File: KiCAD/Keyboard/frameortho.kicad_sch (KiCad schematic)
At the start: 1 part, among them U1 RP2040

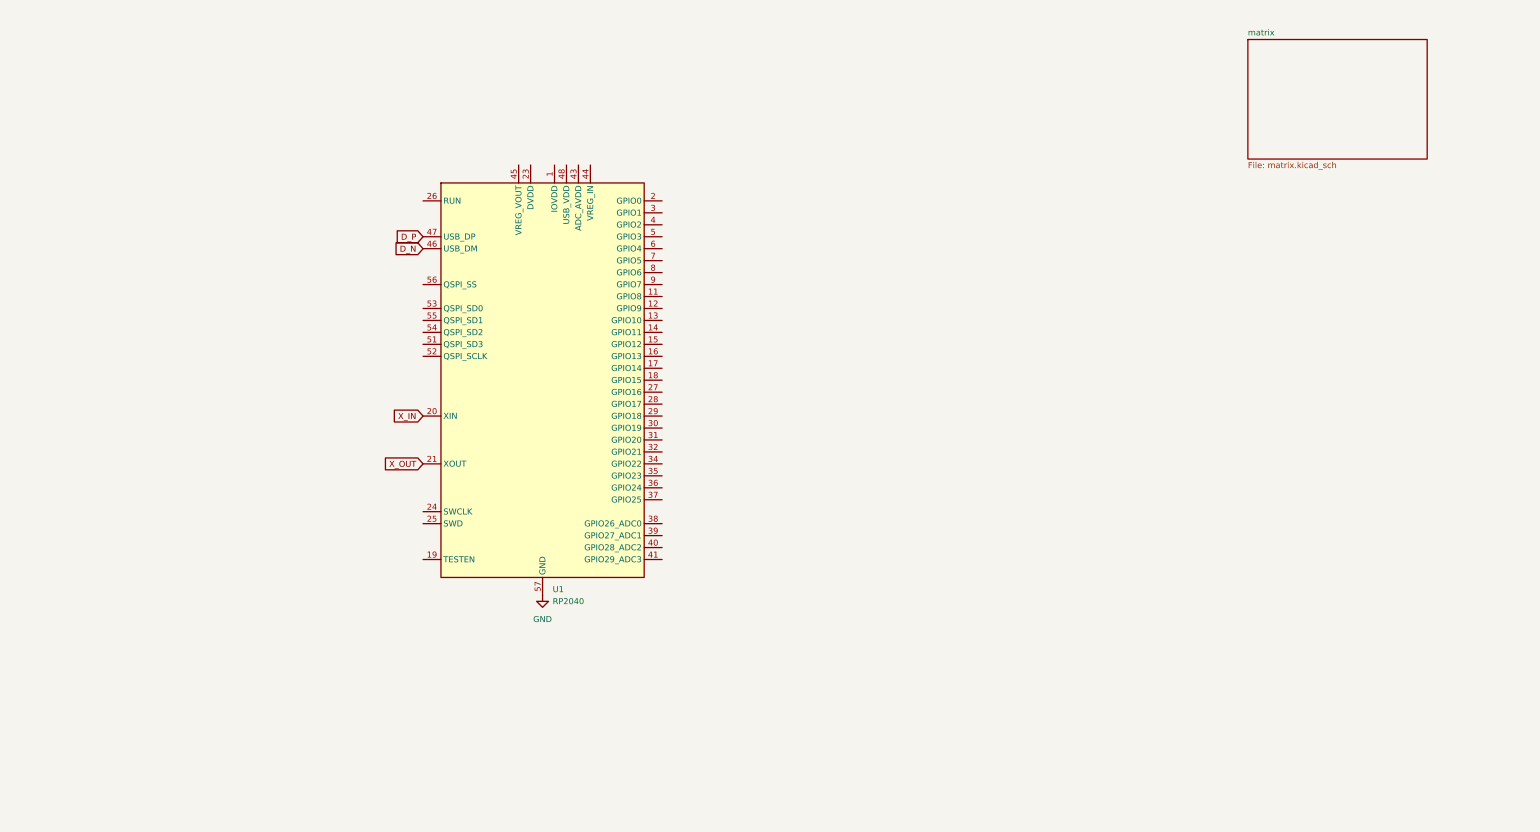
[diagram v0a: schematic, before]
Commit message: start keyboard pcb
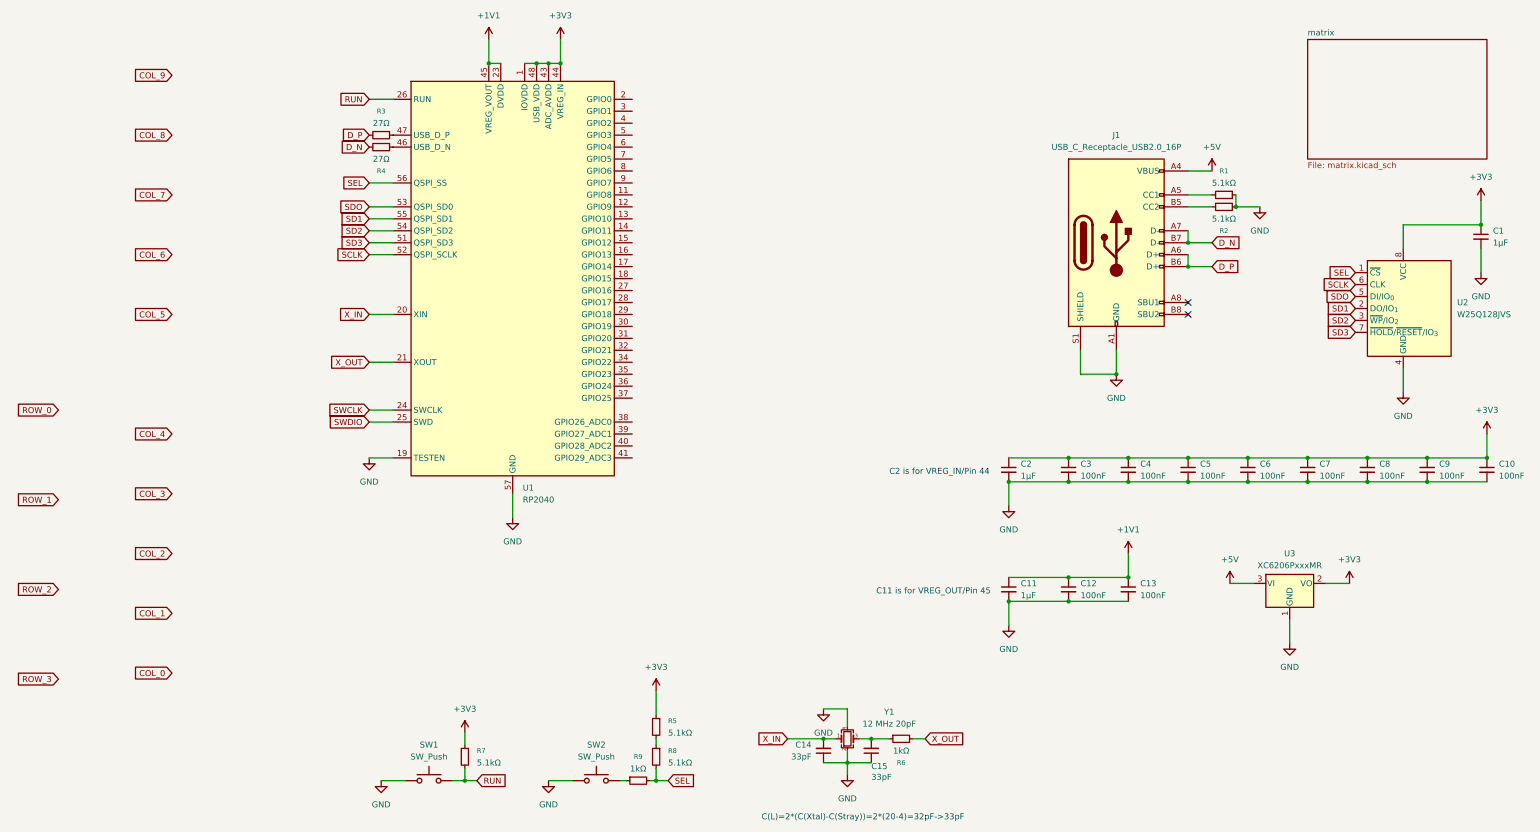
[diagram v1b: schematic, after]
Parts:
- added C1, C11, C2: 1µF, Capacitor_SMD:C_0402_1005Metric, symbol Device:C_Small
- added C10, C12, C13, C3, C4, C5, C6, C7, C8, C9: 100nF, Capacitor_SMD:C_0402_1005Metric, symbol Device:C_Small
- added C14, C15: 33pF, Capacitor_SMD:C_0402_1005Metric, symbol Device:C_Small
- added J1: USB_C_Receptacle_USB2.0_16P, ScottoKeebs_Components:USB_C_HRO_TYPE-C-31-M-14, symbol Connector:USB_C_Receptacle_USB2.0_16P
- added R1, R2, R5, R7, R8: 5.1kΩ, Resistor_SMD:R_0402_1005Metric, symbol Device:R_Small
- added R3, R4: 27Ω, Resistor_SMD:R_0402_1005Metric, symbol Device:R_Small
- added R6, R9: 1kΩ, Resistor_SMD:R_0402_1005Metric, symbol Device:R_Small
- added SW1, SW2: SW_Push, ScottoKeebs_Components:Button_TL3342, symbol Switch:SW_Push
- added U2: W25Q128JVS, Package_SO:SOIC-8_5.3x5.3mm_P1.27mm, symbol Memory_Flash:W25Q128JVS
- added U3: XC6206PxxxMR, Package_TO_SOT_SMD:SOT-23-3, symbol Regulator_Linear:XC6206PxxxMR
- added Y1: 12 MHz 20pF, Crystal:Crystal_SMD_Abracon_ABM3B-4Pin_5.0x3.2mm, symbol Device:Crystal_GND24_Small
- U1: symbol MCU_RaspberryPi:RP2040 -> Custom:RP2040
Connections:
- net D_N: now also J1.A7 (D-), J1.B7 (D-), R4.2; no longer U1.46 (USB_DM)
- net D_P: now also J1.A6 (D+), J1.B6 (D+), R3.2; no longer U1.47 (USB_DP)
- net GND: now also U1.19 (TESTEN), C1.2, C10.2, C11.2, C12.2, C13.2, C14.1, C15.1, C2.2, C3.2, C4.2, C5.2, C6.2, C7.2, C8.2, C9.2, J1.A1 (GND), J1.A12 (GND), J1.B1 (GND), J1.B12 (GND), J1.S1 (SHIELD), R1.1, R2.1, SW1.1, SW2.1, U2.4 (GND), U3.1 (GND), Y1.2, Y1.4
- net X_IN: now also C14.2, Y1.1
- net X_OUT: now also R6.2
- net +3V3: now reaches U1.1 (IOVDD), U1.10 (IOVDD), U1.22 (IOVDD), U1.33 (IOVDD), U1.42 (IOVDD), U1.49 (IOVDD)
- net +3V3: now also U1.43 (ADC_AVDD), U1.44 (VREG_IN), U1.48 (USB_VDD), C1.1, C10.1, C2.1, C3.1, C4.1, C5.1, C6.1, C7.1, C8.1, C9.1, R5.1, R7.1, U2.8 (VCC), U3.2 (VO)
- net +1V1: now reaches U1.23 (DVDD), U1.50 (DVDD)
- net +1V1: now also U1.45 (VREG_VOUT), C11.1, C12.1, C13.1
- net SWCLK: now reaches U1.24 (SWCLK)
- net SWDIO: now reaches U1.25 (SWD)
- net RUN: now reaches U1.26 (RUN)
- net RUN: now also R7.2, SW1.2
- net SD3: now reaches U1.51 (QSPI_SD3)
- net SD3: now also U2.7 (~{HOLD}/~{RESET}/IO_{3})
- net SCLK: now reaches U1.52 (QSPI_SCLK)
- net SCLK: now also U2.6 (CLK)
- net SDO: now reaches U1.53 (QSPI_SD0)
- net SDO: now also U2.5 (DI/IO_{0})
- net SD2: now reaches U1.54 (QSPI_SD2)
- net SD2: now also U2.3 (~{WP}/IO_{2})
- net SD1: now reaches U1.55 (QSPI_SD1)
- net SD1: now also U2.2 (DO/IO_{1})
- net SEL: now reaches U1.56 (QSPI_SS)
- net SEL: now also R8.2, R9.2, U2.1 (~{CS})
- new net: J1.B5 (CC2), R2.2
- new net: R4.1, U1.46 (USB_D_N)
- new net: R3.1, U1.47 (USB_D_P)
- new net: C15.2, R6.1, Y1.3
- new net: R5.2, R8.1
- new net: R9.1, SW2.2
- new net: J1.A5 (CC1), R1.2
- new net +5V: J1.A4 (VBUS), J1.A9 (VBUS), J1.B4 (VBUS), J1.B9 (VBUS), U3.3 (VI)
- no-connect marks 0 -> 2
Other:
- note added: "C(L)=2*(C(Xtal)-C(Stray))=2*(20-4)=32pF->33pF"
- note added: "C11 is for VREG_OUT/Pin 45"
- note added: "C2 is for VREG_IN/Pin 44"
- moved on the sheet: U1

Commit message: mostly finished pcb
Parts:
- removed J1: USB_C_Receptacle_USB2.0_16P, ScottoKeebs_Components:USB_C_HRO_TYPE-C-31-M-14, symbol Connector:USB_C_Receptacle_USB2.0_16P
- removed R1, R2: 5.1kΩ, Resistor_SMD:R_0402_1005Metric, symbol Device:R_Small
- added TP17, TP18, TP19, TP20: TestPoint, TestPoint:TestPoint_Pad_D2.0mm, symbol Connector:TestPoint
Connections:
- net +5V: now also TP17.1
- net COL_0: now also U1.2 (GPIO0)
- net COL_1: now also U1.3 (GPIO1)
- net COL_2: now also U1.4 (GPIO2)
- net COL_3: now also U1.5 (GPIO3)
- net COL_4: now also U1.6 (GPIO4)
- net COL_5: now also U1.31 (GPIO20)
- net COL_6: now also U1.30 (GPIO19)
- net COL_7: now also U1.29 (GPIO18)
- net COL_8: now also U1.28 (GPIO17)
- net COL_9: now also U1.27 (GPIO16)
- net D_N: now also TP19.1
- net D_P: now also TP18.1
- net GND: now also TP20.1
- net ROW_0: now also U1.41 (GPIO29_ADC3)
- net ROW_1: now also U1.40 (GPIO28_ADC2)
- net ROW_2: now also U1.39 (GPIO27_ADC1)
- net ROW_3: now also U1.38 (GPIO26_ADC0)
- net GPIO8: now reaches U1.11 (GPIO8)
- net GPIO9: now reaches U1.12 (GPIO9)
- net GPIO10: now reaches U1.13 (GPIO10)
- net GPIO11: now reaches U1.14 (GPIO11)
- net GPIO12: now reaches U1.15 (GPIO12)
- net GPIO13: now reaches U1.16 (GPIO13)
- net GPIO14: now reaches U1.17 (GPIO14)
- net GPIO15: now reaches U1.18 (GPIO15)
- net GPIO21: now reaches U1.32 (GPIO21)
- net GPIO22: now reaches U1.34 (GPIO22)
- net GPIO23: now reaches U1.35 (GPIO23)
- net GPIO24: now reaches U1.36 (GPIO24)
- net GPIO25: now reaches U1.37 (GPIO25)
- net GPIO5: now reaches U1.7 (GPIO5)
- net GPIO6: now reaches U1.8 (GPIO6)
- net GPIO7: now reaches U1.9 (GPIO7)
- no-connect marks 2 -> 0
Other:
- added sheet pads (pads.kicad_sch)
- note added: "Boot"
- note added: "Buttons"
- note added: "Capacitors"
- note added: "Crystal"
- note added: "Flash"
- note added: "RP2040"
- note added: "Regulator"
- note added: "Reset"
- note added: "USB Pads"
- moved on the sheet: C1, C10, C11, C12, C13, C14, C15, C2, C3, C4, C5, C6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

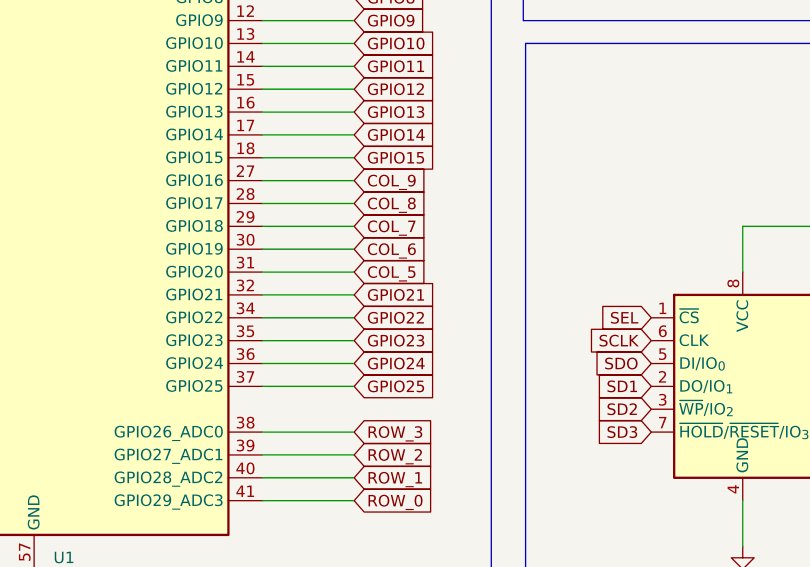
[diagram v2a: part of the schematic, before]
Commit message: idk what i did tbh
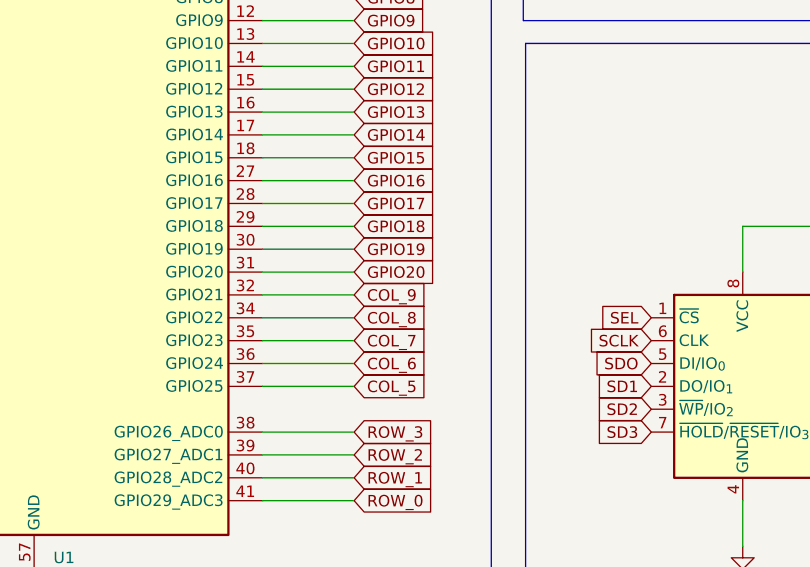
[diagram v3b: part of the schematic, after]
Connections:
- net GPIO21 is gone; now on net COL_9: U1.32 (GPIO21)
- net GPIO22 is gone; now on net COL_8: U1.34 (GPIO22)
- net GPIO23 is gone; now on net COL_7: U1.35 (GPIO23)
- net GPIO24 is gone; now on net COL_6: U1.36 (GPIO24)
- net GPIO25 is gone; now on net COL_5: U1.37 (GPIO25)
- net COL_5: no longer U1.31 (GPIO20)
- net COL_6: no longer U1.30 (GPIO19)
- net COL_7: no longer U1.29 (GPIO18)
- net COL_8: no longer U1.28 (GPIO17)
- net COL_9: no longer U1.27 (GPIO16)
- new net GPIO16: U1.27 (GPIO16)
- new net GPIO17: U1.28 (GPIO17)
- new net GPIO18: U1.29 (GPIO18)
- new net GPIO19: U1.30 (GPIO19)
- new net GPIO20: U1.31 (GPIO20)
